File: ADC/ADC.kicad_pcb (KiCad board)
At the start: 2 copper layers, 38.1 x 63.5 mm, 102 parts, among them P1 CONN_02X05, P2 CONN_02X08, U1 MICA, U2 MICB, U3 TL074, U4 MICC, U5 MICD, U6 AK5703

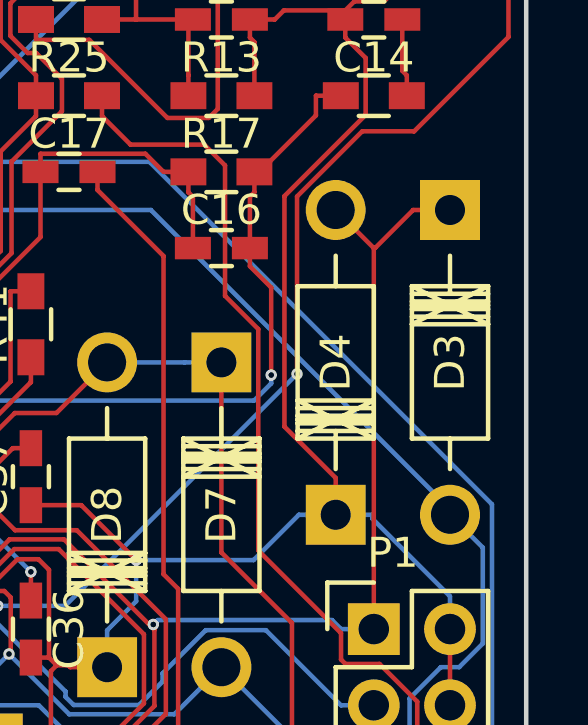
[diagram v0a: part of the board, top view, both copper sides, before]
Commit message: Adjusted 3d models
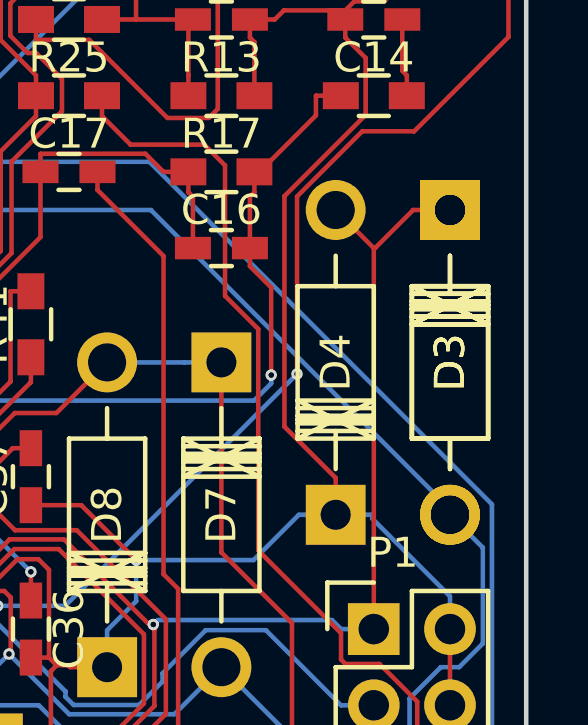
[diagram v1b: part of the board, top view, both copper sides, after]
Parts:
- added D3: D_Schottky, Diodes_ThroughHole:Diode_DO-41_SOD81_Horizontal_RM10, F.Cu at (110.5, 128.3)
